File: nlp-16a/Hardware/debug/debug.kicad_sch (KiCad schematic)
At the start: 15 parts, among them J1 Conn_01x04_Female, J2 Conn_01x04_Male, J3 Conn_01x05_Female, J4 Conn_02x20_Odd_Even, J5 Conn_02x10_Odd_Even, J6 Conn_02x10_Odd_Even, J7 Conn_02x10_Odd_Even, J8 Conn_02x10_Odd_Even, U1 CH32V003F4P6

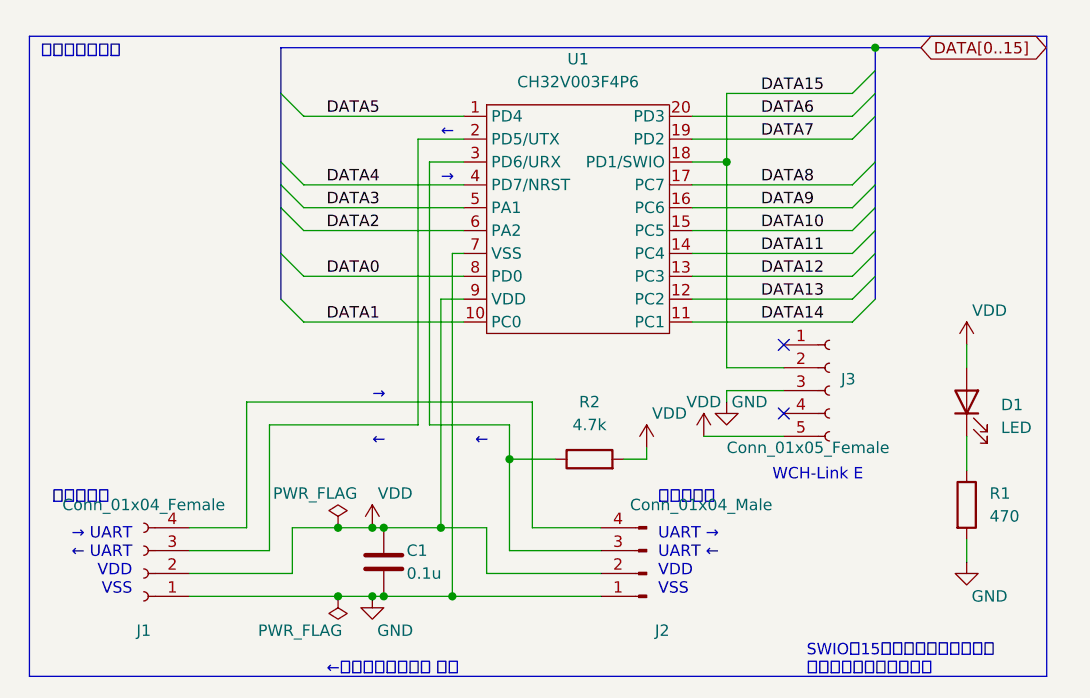
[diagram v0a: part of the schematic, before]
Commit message: デバッガ基板の設計今度こそ完了
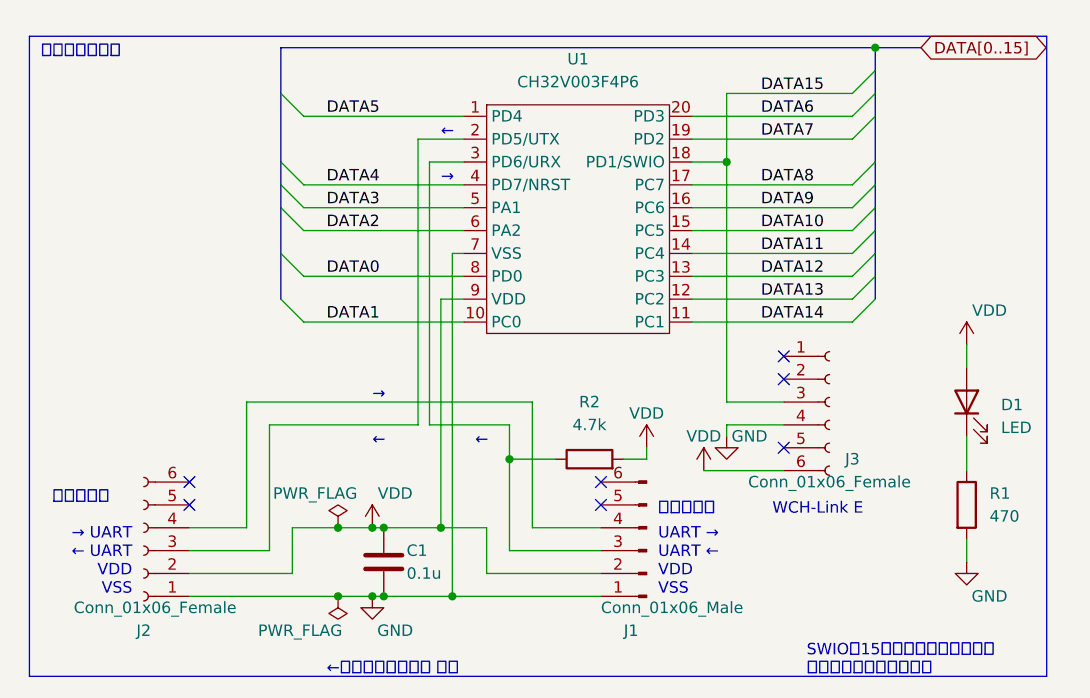
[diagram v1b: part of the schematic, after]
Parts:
- removed J1: Conn_01x04_Female, Connector_PinSocket_2.54mm:PinSocket_1x04_P2.54mm_Horizontal, symbol Connector:Conn_01x04_Female
- removed J2: Conn_01x04_Male, Connector_PinHeader_2.54mm:PinHeader_1x04_P2.54mm_Horizontal, symbol Connector:Conn_01x04_Male
- removed J3: Conn_01x05_Female, Connector_PinSocket_2.54mm:PinSocket_1x05_P2.54mm_Horizontal, symbol Connector:Conn_01x05_Female
- added J1: Conn_01x06_Male, Connector_PinHeader_2.54mm:PinHeader_1x06_P2.54mm_Horizontal, symbol Connector:Conn_01x06_Male
- added J2, J3: Conn_01x06_Female, Connector_PinSocket_2.54mm:PinSocket_1x06_P2.54mm_Horizontal, symbol Connector:Conn_01x06_Female
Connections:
- net DATA15: now also J3.3 (Pin_3)
- net GND: now also J1.1 (Pin_1), J2.1 (Pin_1), J3.4 (Pin_4)
- net VDD: now also J1.2 (Pin_2), J2.2 (Pin_2), J3.6 (Pin_6)
- net at R2.1, U1.3 (PD6/URX): now also J1.3 (Pin_3)
- net at U1.2 (PD5/UTX): now also J2.3 (Pin_3)
- new net: J1.4 (Pin_4), J2.4 (Pin_4)
- no-connect marks 58 -> 63
